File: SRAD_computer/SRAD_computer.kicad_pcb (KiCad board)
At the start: 2 copper layers, 80 x 90 mm, 67 parts, among them J1 Terminal_3, J2 Conn_01x02, J3 UJ20-C-H-G-SMT-1-P16-TR, J4 Terminal_2, J5 Connector_3_Pol, J6 Micro_SD_Card, Q1 MMBT5551L, Q3 FDN340P, U1 NCP1117-3.3_SOT223, U2 W25Q128JVS, U3 RP2040, U4 BME280, U5 MPU-9250, U6 SAM-M8Q-0-10, Y1 Crystal

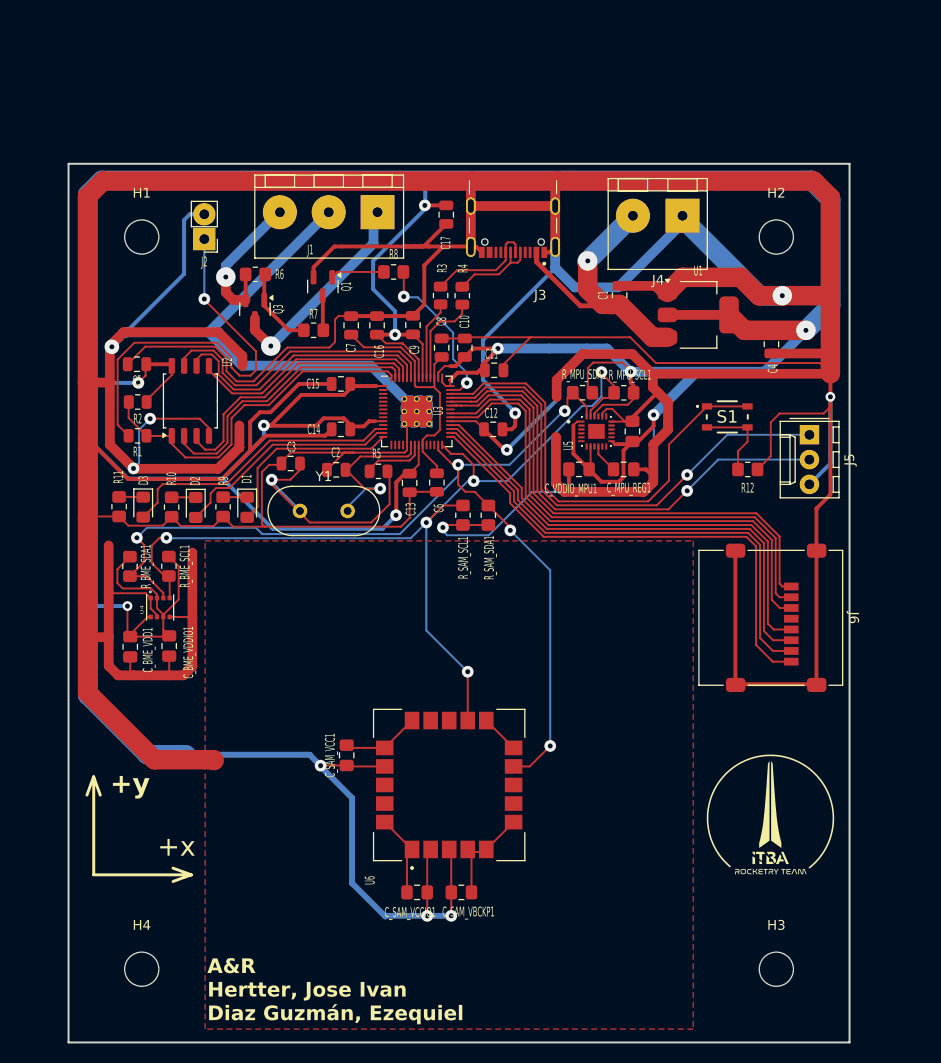
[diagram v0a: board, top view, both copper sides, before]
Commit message: SD layout
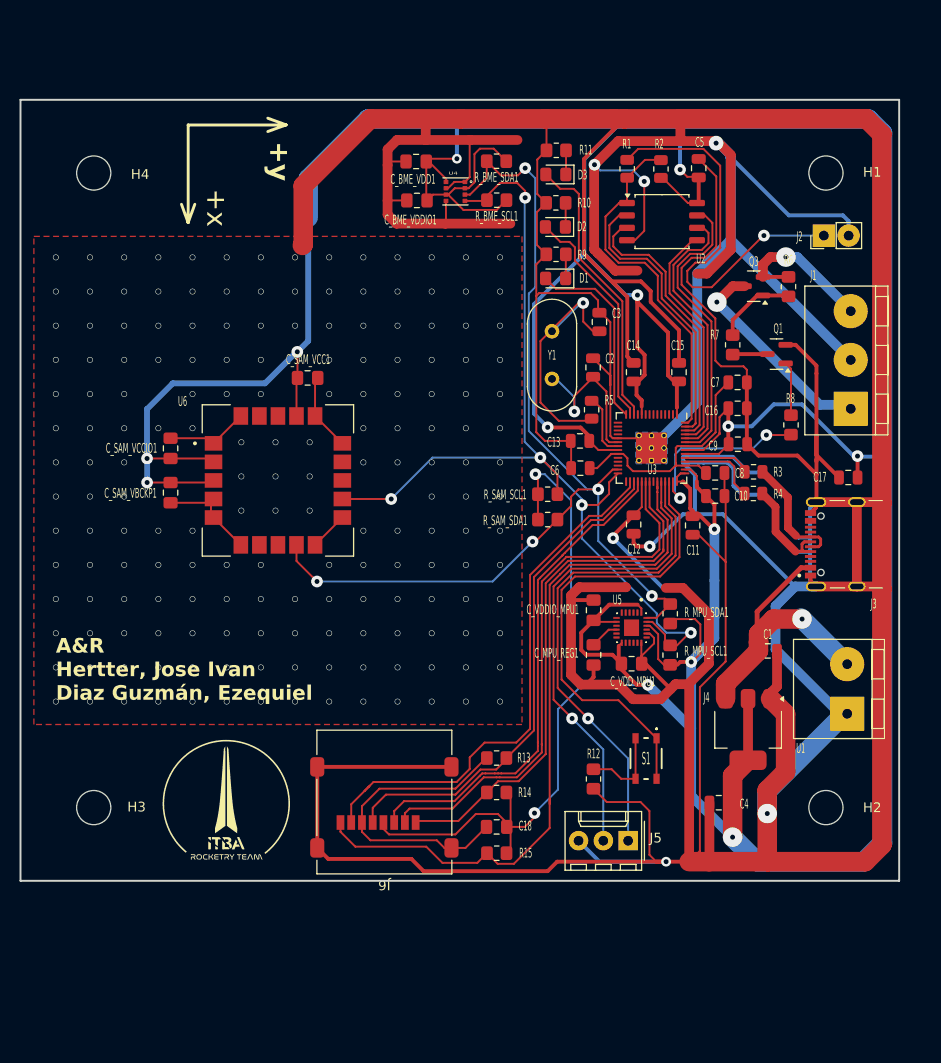
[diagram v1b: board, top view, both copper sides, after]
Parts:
- added C18: 10u, TCLib:C_0805, F.Cu at (93.8, 117.9)
- added R13: R, TCLib:R_0805, F.Cu at (93.8, 110.9)
- added R14: 10k, TCLib:R_0805, F.Cu at (93.8, 114.4)
- added R15: 10k, TCLib:R_0805, F.Cu at (93.9, 120.6)
- moved H4 81.7 mm to (52.6, 50.9), turned to -90 degrees
- moved H3 71.9 mm to (52.6, 115.9), turned to -90 degrees
- moved H1 70.4 mm to (127.6, 50.9), turned to -90 degrees
- moved J2 63.5 mm to (127.4, 57.4), turned to 90 degrees
- moved C5 60.9 mm to (114.5, 50.5), turned to 90 degrees
- moved R2 58.7 mm to (110.7, 50.5), turned to 90 degrees
- moved H2 58.7 mm to (127.6, 115.9), turned to -90 degrees
- moved R11 57.8 mm to (100.0, 48.6), turned to 180 degrees
- moved C_BME_VDD1 57.7 mm to (85.6, 49.8), turned to 180 degrees
- moved R1 57.1 mm to (107.2, 50.5), turned to 90 degrees
- moved R_BME_SDA1 56.0 mm to (93.8, 49.7), turned to 180 degrees
- moved G*** 55.8 mm to (66.2, 115.7)
- moved R6 54.6 mm to (123.8, 62.6), turned to -90 degrees
- moved D3 54.3 mm to (99.9, 51.1), turned to 180 degrees
- moved J4 53.7 mm to (129.8, 106.3), turned to 90 degrees
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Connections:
- J6 pad 4: unconnected-(J6-VDD-Pad4) -> +3V3
- J6 pad 6: /SD_VSS -> GND
- U3 pad 29: /SD_DAT1 -> /GPIO18
- U3 pad 31: /SD_VSS -> /SD_CLK
- U3 pad 32: /SD_CLK -> /SD_CMD
- U3 pad 34: /SD_CMD -> /SD_DAT3
- U3 pad 35: /SD_DAT3 -> /SD_DAT2
- U3 pad 37: /SD_DAT2 -> /SD_DAT1
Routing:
- net GND: track 852.7 -> 945.8 mm, vias 6 -> 185
- net /SD_VSS: track 49.8 -> 0.00 mm
- net +3V3: track 548.5 -> 589.6 mm, vias 15 -> 16
- net /SD_DAT1: track 51.0 -> 72.8 mm
- net /SD_DAT0: track 50.4 -> 55.9 mm
- net /SD_DAT3: track 52.3 -> 56.8 mm
- net /SD_DAT2: track 51.6 -> 55.3 mm
- net /SD_CLK: track 49.1 -> 51.8 mm
- net /power_cam: track 16.8 -> 19.4 mm
- net /SD_CMD: track 52.9 -> 50.9 mm
- net /USB_D-: track 8.92 -> 10.7 mm
- net Net-(U3-USB_DP): track 8.54 -> 6.93 mm
- net Net-(U3-USB_DM): track 9.73 -> 8.44 mm
- net /USB_D+: track 11.4 -> 12.5 mm
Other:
- board size 80 x 90 mm -> 90 x 80 mm

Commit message: .
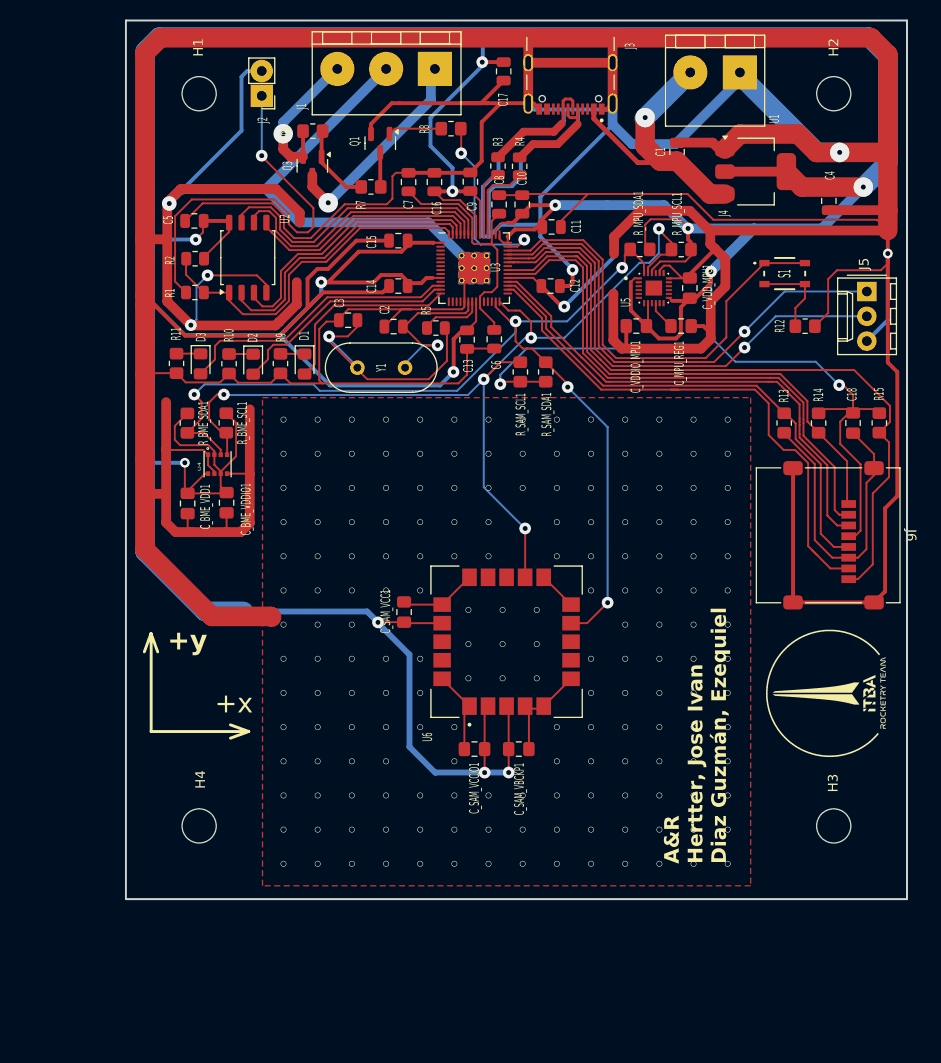
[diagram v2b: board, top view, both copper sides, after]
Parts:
- moved H3 75.8 mm to (128.4, 117.8), turned to 0 degrees
- moved H2 73.1 mm to (128.4, 42.8), turned to 0 degrees
- moved H4 67.7 mm to (63.4, 117.8), turned to 0 degrees
- moved J4 66.6 mm to (118.8, 40.6), turned to 180 degrees
- moved H1 64.7 mm to (63.4, 42.8), turned to 0 degrees
- moved G*** 63.0 mm to (128.2, 104.2), turned to 90 degrees
- moved C4 62.7 mm to (127.9, 53.8), turned to -90 degrees
- moved J5 61.3 mm to (131.8, 63.1), turned to -90 degrees
- moved J3 61.0 mm to (101.4, 37.1), turned to 180 degrees
- moved J2 59.3 mm to (69.8, 43.0), turned to 180 degrees
- moved R15 59.0 mm to (133.1, 76.5), turned to -90 degrees
- moved U1 57.1 mm to (120.4, 50.8), turned to 0 degrees
- moved C18 55.2 mm to (130.4, 76.6), turned to -90 degrees
- moved J1 55.0 mm to (87.5, 40.3), turned to 180 degrees
- moved C17 54.6 mm to (94.6, 40.5), turned to -90 degrees
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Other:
- board size 90 x 80 mm -> 80 x 90 mm
